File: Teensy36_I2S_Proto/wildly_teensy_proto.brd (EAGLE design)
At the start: 87.6 x 77.5 mm, 42 parts, among them J1 61300311121, J2 61300311121, T1 2N2222A, T2 2N2222A, T3 2N2222A, T4 2N2222A

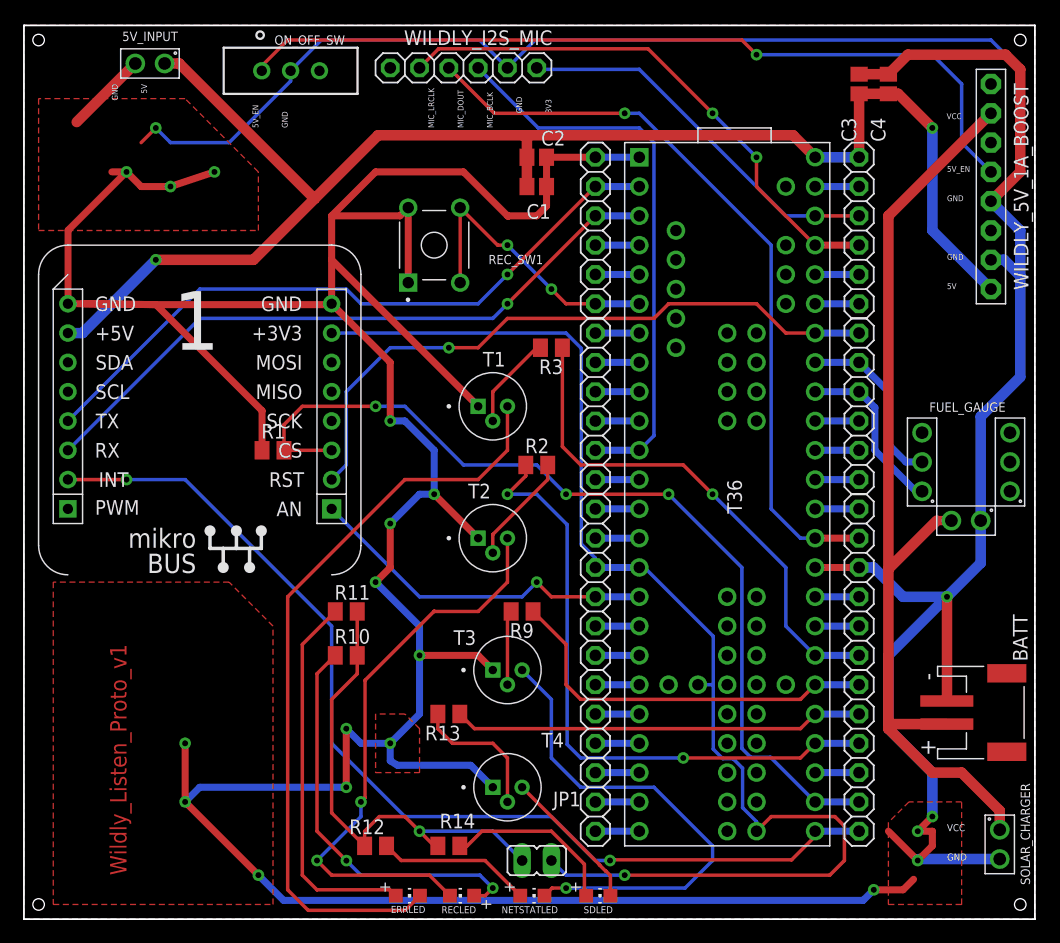
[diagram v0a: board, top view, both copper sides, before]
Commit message: Added new transistor BC847 along with some 0R reistors
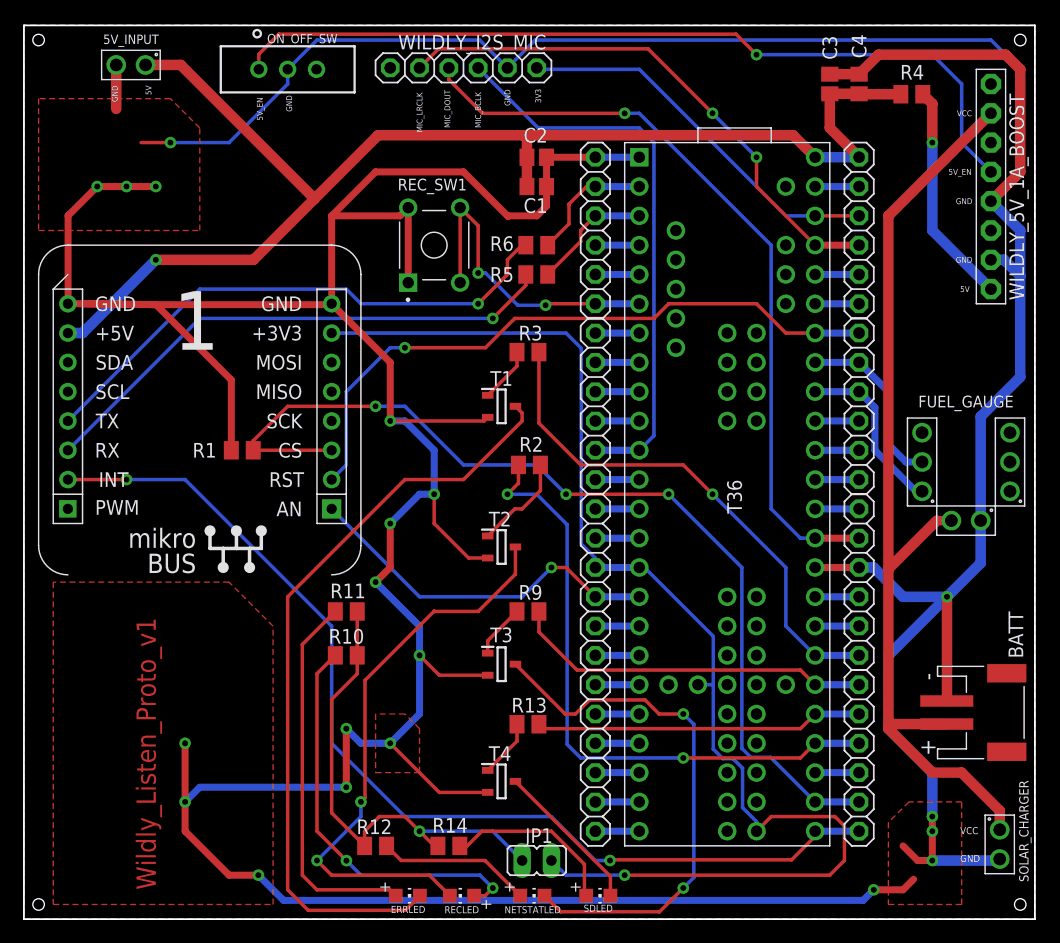
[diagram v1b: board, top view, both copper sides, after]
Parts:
- added R4, R5, R6: 0R, adafruit:M0805
- T1, T2, T3, T4: value 2N2222A -> BC847BLT1G; device 2N2222A:TO127P584H533-3 -> BC847BLT1G:SOT96P237X111-3N
- moved R13 6.92 mm to (43.7, 16.9)
- moved R1 2.67 mm to (18.9, 40.6)
- moved C3 2.54 mm to (69.8, 72.4)
- moved C4 2.54 mm to (72.4, 72.4)
- moved R3 2.07 mm to (43.7, 49.1)
- moved 5V_INPUT 1.66 mm to (9.27, 74.0)
- moved T2 1.08 mm to (41.4, 32.3)
- moved T1 0.76 mm to (41.4, 44.5)
- moved T4 0.72 mm to (41.4, 11.9)
- moved T3 0.72 mm to (41.4, 22.1)
- moved R2 0.64 mm to (43.8, 39.4)
- moved R9 0.51 mm to (43.7, 26.7)
- moved ON_OFF_SW 0.28 mm to (22.9, 73.7)
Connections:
- net 5V_SUPPLY: now also R4.1, R4.2
- net GND: now also T1.2, T2.2, T3.2, T4.2; no longer T1.1, T2.1, T3.1, T4.1
- net N$11: now also T4.1; no longer T4.2
- net N$3: now also T2.1; no longer T2.2
- net N$7: now also T3.1; no longer T3.2
- net N$8: now also T1.1; no longer T1.2
- net RX_OF_GSM: now also R5.1, R5.2
- net TX_OF_GSM: now also R6.1, R6.2
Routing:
- net GND: track 544.4 -> 524.5 mm
- net SDLED: track 35.7 -> 28.4 mm
- net N$11: track 12.2 -> 5.05 mm
- net 5V_SUPPLY: track 128.1 -> 132.6 mm
- net RTS_OF_GSM: track 80.2 -> 84.8 mm
- net N$5: track 42.9 -> 46.7 mm, vias 1 -> 2
- net N$8: track 8.25 -> 4.79 mm
- net NETSTATLED: track 34.0 -> 31.4 mm
- net PWM3: track 25.5 -> 28.0 mm
- net N$7: track 6.48 -> 4.67 mm
- net N$3: track 9.59 -> 8.42 mm
- net 5V_EN: track 72.3 -> 73.4 mm
- net NET_STAT: track 30.9 -> 31.9 mm
- net RX_OF_GSM: track 57.9 -> 57.2 mm
- net N$1: track 12.6 -> 13.3 mm
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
